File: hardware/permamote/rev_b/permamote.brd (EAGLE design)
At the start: 27 x 60 mm, 126 parts, among them J1 TC2030-JLINK-NL, J5 MICRO_USB_B_HIROSE_ZX62R-B-5P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, Q1 PMDXB950UPEL, Q10 PMDXB950UPEL, Q2 PMDXB950UPEL, Q3 PMDXB950UPEL, Q4 PMDXB950UPEL, Q5 PMDXB950UPEL, Q6 PMDXB950UPEL, Q7 PMDXB950UPEL, Q8 PMDXB950UPEL, U1 AB1815-T3, U10 NRF52840, U11 SI7021-A20-GM1, U12 TCS34725, U2 BQ25505, U3 EKMB1101111, U4 FT232RQ, U6 LIS2DW12, U7 MAX17222, U8 MAX44009, U9 MS5637-02BA03, X1 32MHz, X3 32.768kHz, X4 ABS07-32.768KHZ-7-T

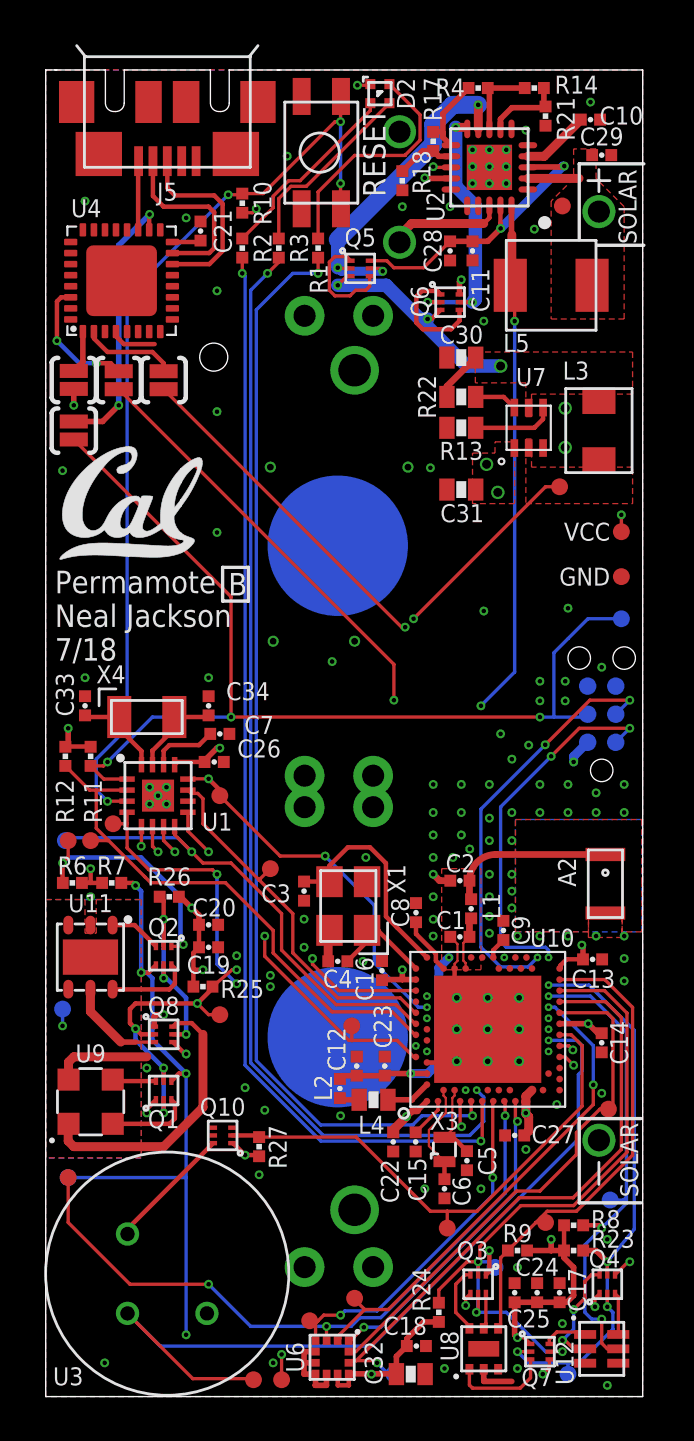
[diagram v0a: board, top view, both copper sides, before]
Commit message: Revert "Move jtag connector to back"
This reverts commit 0289d5f44ae80c2e7a408d73da812219b95e3e35.

start rev c
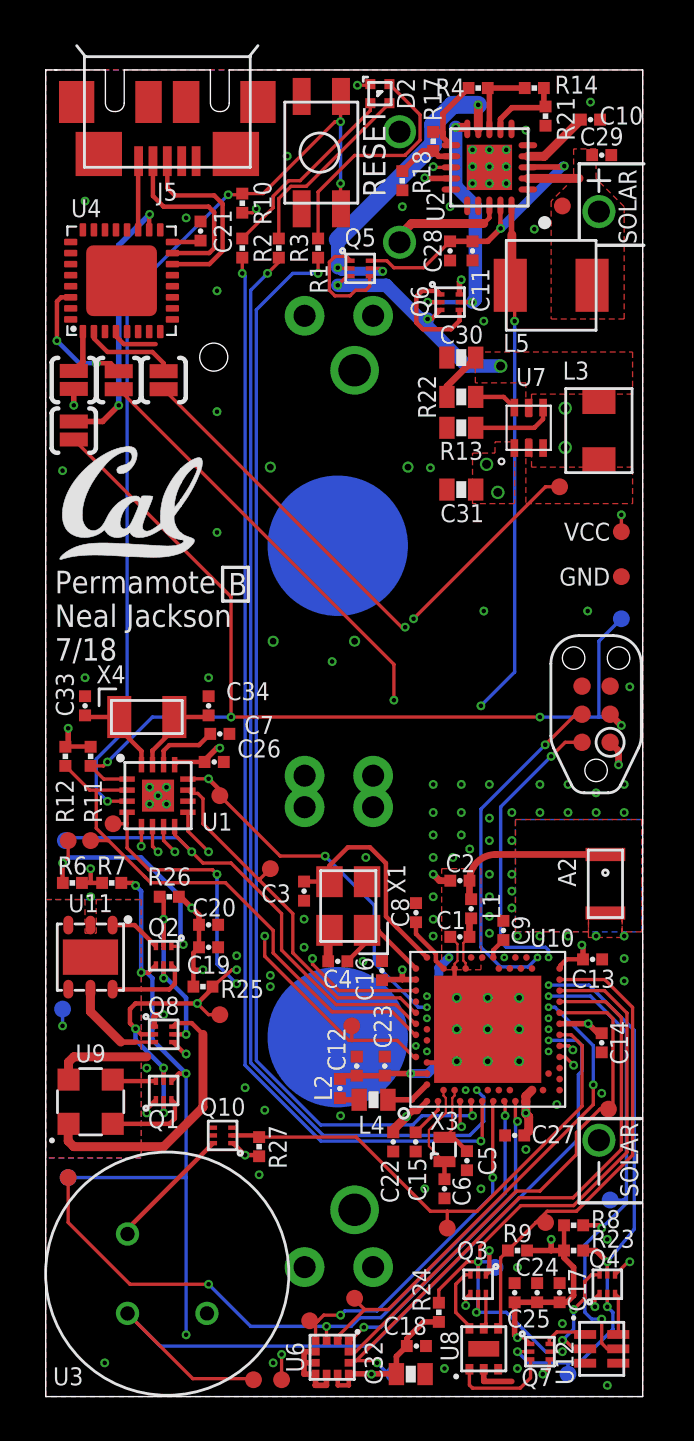
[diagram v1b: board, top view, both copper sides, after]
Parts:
- moved J1 0.25 mm to (24.9, 30.9), flipped to the top
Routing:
- net SWDCLK: track 19.0 -> 15.7 mm, vias 3 -> 2
- net SWDIO: track 17.0 -> 13.6 mm, vias 3 -> 2
- net !RST: track 64.9 -> 65.5 mm, vias 4 -> 5
- net GND: vias 117 -> 110
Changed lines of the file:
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@@
 <attribute name="NAME" x="7.62" y="21.717" size="0.8128" layer="25" font="vector" ratio="12" align="bottom-center"/>
 </element>
-<element name="J1" library="connector" package="TC2030-IDC-NL" value="TC2030-JLINK-NL" x="25.146" y="30.861" smashed="yes" rot="MR90">
-<attribute name="VALUE" x="19.1135" y="30.861" size="1.016" layer="28" font="vector" ratio="12" rot="MR90" align="bottom-center"/>
+<element name="J1" library="connector" package="TC2030-IDC-NL" value="TC2030-JLINK-NL" x="24.892" y="30.861" smashed="yes" rot="R90">
+<attribute name="VALUE" x="30.9245" y="30.861" size="1.016" layer="27" font="vector" ratio="12" rot="R90" align="bottom-center"/>
 </element>
 <element name="R23" library="passives" package="0402_RES" value="100M" x="23.876" y="6.604" smashed="yes" rot="R180">
@@
 <wire x1="17.242" y1="14.61" x2="16.51" y2="14.61" width="0.254" layer="1"/>
 <wire x1="16.51" y1="14.61" x2="15.43106875" y2="14.61" width="0.254" layer="1"/>
+<wire x1="18.242" y1="19.86" x2="18.2279625" y2="19.8740375" width="0.2032" layer="1"/>
 <via x="16.51" y="14.61" extent="1-16" drill="0.2032"/>
 <via x="18.242" y="19.86" extent="1-16" drill="0.1524"/>
@@
 <contactref element="C21" pad="2"/>
 <contactref element="J5" pad="5"/>
+<wire x1="18.534" y1="18.6392" x2="18.5288" y2="18.634" width="0.1016" layer="1"/>
 <via x="18.288" y="53.816" extent="1-16" drill="0.2032"/>
 <via x="6.35" y="53.308" extent="1-16" drill="0.2032"/>
@@
 <wire x1="3.18" y1="47.95599375" x2="3.53639375" y2="47.5996" width="0.2032" layer="1"/>
 <wire x1="3.18" y1="48.167" x2="3.18" y2="47.95599375" width="0.2032" layer="1"/>
+<wire x1="3.53639375" y1="47.5996" x2="4.9733" y2="47.5996" width="0.2032" layer="1"/>
 <via x="11.684" y="21.59" extent="1-16" drill="0.2032"/>
 <via x="11.684" y="20.32" extent="1-16" drill="0.2032"/>
@@
 <via x="17.399" y="42.005" extent="1-16" drill="0.2032"/>
 <via x="19.812" y="35.528" extent="1-16" drill="0.2032"/>
-<via x="23.622" y="35.655" extent="1-16" drill="0.2032"/>
-<via x="23.495" y="32.353" extent="1-16" drill="0.2032"/>
+<via x="24.511" y="35.528" extent="1-16" drill="0.2032"/>
+<via x="26.416" y="32.099" extent="1-16" drill="0.2032"/>
 <contactref element="C9" pad="2"/>
 <via x="21.336" y="20.828" extent="1-16" drill="0.2032"/>
@@
 <wire x1="17.526" y1="23.622" x2="17.815" y2="23.333" width="0.3048" layer="1"/>
 <wire x1="17.815" y1="23.333" x2="18.29893125" y2="23.333" width="0.3048" layer="1"/>
-<via x="23.495" y="31.464" extent="1-16" drill="0.2032"/>
-<via x="25.146" y="32.988" extent="1-16" drill="0.2032"/>
-<via x="22.352" y="32.353" extent="1-16" drill="0.2032"/>
-<via x="22.352" y="31.464" extent="1-16" drill="0.2032"/>
-<wire x1="3.53639375" y1="47.5996" x2="4.9276" y2="47.5996" width="0.2032" layer="1"/>
-<via x="21.082" y="28.829" extent="1-16" drill="0.2032"/>
-<via x="21.844" y="29.464" extent="1-16" drill="0.2032"/>
-<via x="20.574" y="29.972" extent="1-16" drill="0.2032"/>
 </signal>
 <signal name="N$8">
@@
 <wire x1="6.93293125" y1="21.336" x2="6.93293125" y2="21.76906875" width="0.254" layer="1"/>
 <wire x1="6.93293125" y1="21.76906875" x2="6.604" y2="22.098" width="0.254" layer="1"/>
-<via x="23.876" y="28.702" extent="1-16" drill="0.2032"/>
+<via x="25.908" y="28.575" extent="1-16" drill="0.2032"/>
 <wire x1="16.129" y1="19.304" x2="16.129" y2="18.86" width="0.254" layer="1"/>
 <wire x1="16.33093125" y1="2.286" x2="16.33093125" y2="2.61493125" width="0.254" layer="1"/>
@@
 <wire x1="13.97" y1="34.163" x2="15.748" y2="34.163" width="0.8128" layer="15"/>
 <via x="10.287" y="34.163" extent="1-16" drill="0.3048"/>
+<wire x1="25.908" y1="28.575" x2="25.908" y2="29.21" width="0.3048" layer="1"/>
+<wire x1="25.908" y1="29.21" x2="25.527" y2="29.591" width="0.3048" layer="1"/>
 <wire x1="15.748" y1="34.163" x2="16.383" y2="33.528" width="0.8128" layer="15"/>
-<wire x1="24.511" y1="29.591" x2="23.876" y2="28.956" width="0.4064" layer="16"/>
-<wire x1="23.876" y1="28.956" x2="23.876" y2="28.702" width="0.4064" layer="16"/>
+<wire x1="16.383" y1="33.528" x2="16.4338" y2="33.528" width="0.8128" layer="15"/>
 </signal>
 <signal name="N$12">
@@
 <via x="22.742" y="16.61" extent="1-16" drill="0.1524"/>
 <contactref element="SJ3" pad="1"/>
+<via x="26.035" y="30.353" extent="1-16" drill="0.2032"/>
 <wire x1="2.032" y1="28.52293125" x2="2.62693125" y2="27.928" width="0.1524" layer="1"/>
 <wire x1="2.62693125" y1="27.928" x2="3.68" y2="27.928" width="0.1524" layer="1"/>
@@
 <wire x1="1.27" y1="43.2871" x2="8.382" y2="36.1751" width="0.1524" layer="1"/>
 <wire x1="8.382" y1="36.1751" x2="8.382" y2="30.734" width="0.1524" layer="1"/>
+<wire x1="26.035" y1="35.179" x2="25.019" y2="34.163" width="0.1524" layer="16"/>
+<wire x1="25.527" y1="30.861" x2="26.035" y2="30.353" width="0.3048" layer="1"/>
+<wire x1="22.352" y1="30.734" x2="25.019" y2="30.734" width="0.1524" layer="16"/>
+<wire x1="25.019" y1="30.734" x2="25.654" y2="30.734" width="0.1524" layer="16"/>
+<wire x1="25.654" y1="30.734" x2="26.035" y2="30.353" width="0.1524" layer="16"/>
+<wire x1="25.019" y1="34.163" x2="25.019" y2="30.734" width="0.1524" layer="16"/>
 <wire x1="22.742" y1="16.61" x2="22.91" y2="16.61" width="0.1524" layer="15"/>
-<wire x1="22.352" y1="30.734" x2="22.987" y2="30.734" width="0.1524" layer="16"/>
-<wire x1="22.987" y1="30.734" x2="24.384" y2="30.734" width="0.1524" layer="16"/>
-<wire x1="24.384" y1="30.734" x2="24.511" y2="30.861" width="0.1524" layer="16"/>
-<wire x1="22.987" y1="33.6422375" x2="23.6347625" y2="34.29" width="0.1524" layer="16"/>
-<wire x1="22.987" y1="30.734" x2="22.987" y2="33.6422375" width="0.1524" layer="16"/>
-<wire x1="23.6347625" y1="34.29" x2="24.5237625" y2="35.179" width="0.1524" layer="16"/>
-<wire x1="24.5237625" y1="35.179" x2="26.035" y2="35.179" width="0.1524" layer="16"/>
 </signal>
 <signal name="!RTC_IRQ1">
@@
 <wire x1="20.574" y1="26.67" x2="20.574" y2="20.574" width="0.1524" layer="16"/>
 <wire x1="20.574" y1="20.574" x2="20.828" y2="20.32" width="0.1524" layer="16"/>
-<wire x1="22.86" y1="28.956" x2="24.13" y2="30.226" width="0.1524" layer="1"/>
-<wire x1="24.13" y1="30.226" x2="26.416" y2="30.226" width="0.1524" layer="1"/>
-<via x="26.416" y="30.226" extent="1-16" drill="0.2032"/>
-<wire x1="26.416" y1="30.226" x2="25.781" y2="29.591" width="0.1524" layer="16"/>
+<wire x1="22.86" y1="28.956" x2="23.495" y2="29.591" width="0.1524" layer="1"/>
+<wire x1="23.495" y1="29.591" x2="24.257" y2="29.591" width="0.1524" layer="1"/>
 </signal>
 <signal name="RTC_CS">
@@
 <wire x1="19.685" y1="20.32" x2="19.685" y2="26.57126875" width="0.1524" layer="16"/>
 <wire x1="19.685" y1="26.57126875" x2="22.591865625" y2="29.478134375" width="0.1524" layer="16"/>
-<wire x1="22.591865625" y1="29.478134375" x2="24.60973125" y2="31.496" width="0.1524" layer="1"/>
-<wire x1="24.60973125" y1="31.496" x2="26.416" y2="31.496" width="0.1524" layer="1"/>
-<via x="26.416" y="31.496" extent="1-16" drill="0.2032"/>
-<wire x1="26.416" y1="31.496" x2="25.781" y2="30.861" width="0.1524" layer="16"/>
+<wire x1="22.591865625" y1="29.478134375" x2="23.97473125" y2="30.861" width="0.1524" layer="1"/>
+<wire x1="23.97473125" y1="30.861" x2="24.257" y2="30.861" width="0.1524" layer="1"/>
 </signal>
 <signal name="N$41">

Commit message: Move jtag connector to back
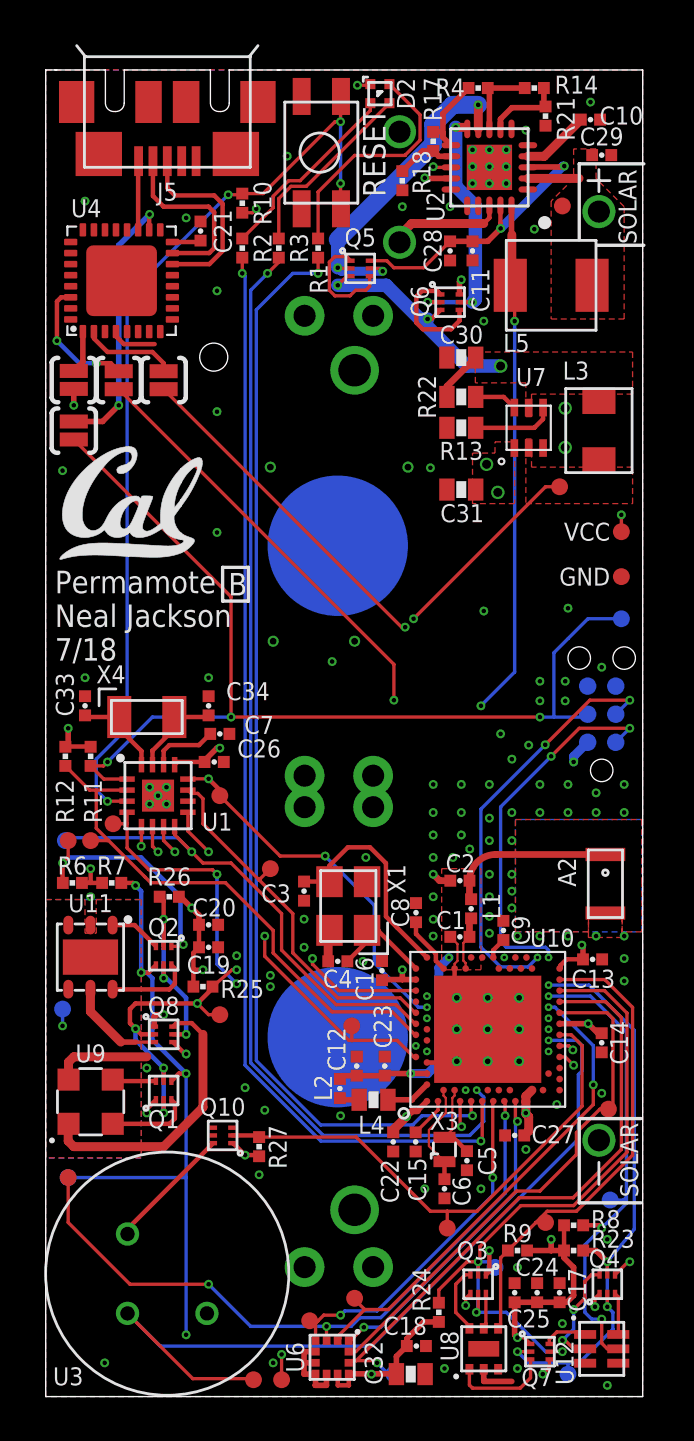
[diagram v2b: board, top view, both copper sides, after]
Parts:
- moved J1 0.25 mm to (25.1, 30.9), flipped to the bottom
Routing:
- net SWDCLK: track 15.7 -> 19.0 mm, vias 2 -> 3
- net SWDIO: track 13.6 -> 17.0 mm, vias 2 -> 3
- net !RST: track 65.5 -> 64.9 mm, vias 5 -> 4
- net GND: vias 110 -> 117
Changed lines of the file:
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@@
 <attribute name="NAME" x="7.62" y="21.717" size="0.8128" layer="25" font="vector" ratio="12" align="bottom-center"/>
 </element>
-<element name="J1" library="connector" package="TC2030-IDC-NL" value="TC2030-JLINK-NL" x="24.892" y="30.861" smashed="yes" rot="R90">
-<attribute name="VALUE" x="30.9245" y="30.861" size="1.016" layer="27" font="vector" ratio="12" rot="R90" align="bottom-center"/>
+<element name="J1" library="connector" package="TC2030-IDC-NL" value="TC2030-JLINK-NL" x="25.146" y="30.861" smashed="yes" rot="MR90">
+<attribute name="VALUE" x="19.1135" y="30.861" size="1.016" layer="28" font="vector" ratio="12" rot="MR90" align="bottom-center"/>
 </element>
 <element name="R23" library="passives" package="0402_RES" value="100M" x="23.876" y="6.604" smashed="yes" rot="R180">
@@
 <wire x1="17.242" y1="14.61" x2="16.51" y2="14.61" width="0.254" layer="1"/>
 <wire x1="16.51" y1="14.61" x2="15.43106875" y2="14.61" width="0.254" layer="1"/>
-<wire x1="18.242" y1="19.86" x2="18.2279625" y2="19.8740375" width="0.2032" layer="1"/>
 <via x="16.51" y="14.61" extent="1-16" drill="0.2032"/>
 <via x="18.242" y="19.86" extent="1-16" drill="0.1524"/>
@@
 <contactref element="C21" pad="2"/>
 <contactref element="J5" pad="5"/>
-<wire x1="18.534" y1="18.6392" x2="18.5288" y2="18.634" width="0.1016" layer="1"/>
 <via x="18.288" y="53.816" extent="1-16" drill="0.2032"/>
 <via x="6.35" y="53.308" extent="1-16" drill="0.2032"/>
@@
 <wire x1="3.18" y1="47.95599375" x2="3.53639375" y2="47.5996" width="0.2032" layer="1"/>
 <wire x1="3.18" y1="48.167" x2="3.18" y2="47.95599375" width="0.2032" layer="1"/>
-<wire x1="3.53639375" y1="47.5996" x2="4.9733" y2="47.5996" width="0.2032" layer="1"/>
 <via x="11.684" y="21.59" extent="1-16" drill="0.2032"/>
 <via x="11.684" y="20.32" extent="1-16" drill="0.2032"/>
@@
 <via x="17.399" y="42.005" extent="1-16" drill="0.2032"/>
 <via x="19.812" y="35.528" extent="1-16" drill="0.2032"/>
-<via x="24.511" y="35.528" extent="1-16" drill="0.2032"/>
-<via x="26.416" y="32.099" extent="1-16" drill="0.2032"/>
+<via x="23.622" y="35.655" extent="1-16" drill="0.2032"/>
+<via x="23.495" y="32.353" extent="1-16" drill="0.2032"/>
 <contactref element="C9" pad="2"/>
 <via x="21.336" y="20.828" extent="1-16" drill="0.2032"/>
@@
 <wire x1="17.526" y1="23.622" x2="17.815" y2="23.333" width="0.3048" layer="1"/>
 <wire x1="17.815" y1="23.333" x2="18.29893125" y2="23.333" width="0.3048" layer="1"/>
+<via x="23.495" y="31.464" extent="1-16" drill="0.2032"/>
+<via x="25.146" y="32.988" extent="1-16" drill="0.2032"/>
+<via x="22.352" y="32.353" extent="1-16" drill="0.2032"/>
+<via x="22.352" y="31.464" extent="1-16" drill="0.2032"/>
+<wire x1="3.53639375" y1="47.5996" x2="4.9276" y2="47.5996" width="0.2032" layer="1"/>
+<via x="21.082" y="28.829" extent="1-16" drill="0.2032"/>
+<via x="21.844" y="29.464" extent="1-16" drill="0.2032"/>
+<via x="20.574" y="29.972" extent="1-16" drill="0.2032"/>
 </signal>
 <signal name="N$8">
@@
 <wire x1="6.93293125" y1="21.336" x2="6.93293125" y2="21.76906875" width="0.254" layer="1"/>
 <wire x1="6.93293125" y1="21.76906875" x2="6.604" y2="22.098" width="0.254" layer="1"/>
-<via x="25.908" y="28.575" extent="1-16" drill="0.2032"/>
+<via x="23.876" y="28.702" extent="1-16" drill="0.2032"/>
 <wire x1="16.129" y1="19.304" x2="16.129" y2="18.86" width="0.254" layer="1"/>
 <wire x1="16.33093125" y1="2.286" x2="16.33093125" y2="2.61493125" width="0.254" layer="1"/>
@@
 <wire x1="13.97" y1="34.163" x2="15.748" y2="34.163" width="0.8128" layer="15"/>
 <via x="10.287" y="34.163" extent="1-16" drill="0.3048"/>
-<wire x1="25.908" y1="28.575" x2="25.908" y2="29.21" width="0.3048" layer="1"/>
-<wire x1="25.908" y1="29.21" x2="25.527" y2="29.591" width="0.3048" layer="1"/>
 <wire x1="15.748" y1="34.163" x2="16.383" y2="33.528" width="0.8128" layer="15"/>
-<wire x1="16.383" y1="33.528" x2="16.4338" y2="33.528" width="0.8128" layer="15"/>
+<wire x1="24.511" y1="29.591" x2="23.876" y2="28.956" width="0.4064" layer="16"/>
+<wire x1="23.876" y1="28.956" x2="23.876" y2="28.702" width="0.4064" layer="16"/>
 </signal>
 <signal name="N$12">
@@
 <via x="22.742" y="16.61" extent="1-16" drill="0.1524"/>
 <contactref element="SJ3" pad="1"/>
-<via x="26.035" y="30.353" extent="1-16" drill="0.2032"/>
 <wire x1="2.032" y1="28.52293125" x2="2.62693125" y2="27.928" width="0.1524" layer="1"/>
 <wire x1="2.62693125" y1="27.928" x2="3.68" y2="27.928" width="0.1524" layer="1"/>
@@
 <wire x1="1.27" y1="43.2871" x2="8.382" y2="36.1751" width="0.1524" layer="1"/>
 <wire x1="8.382" y1="36.1751" x2="8.382" y2="30.734" width="0.1524" layer="1"/>
-<wire x1="26.035" y1="35.179" x2="25.019" y2="34.163" width="0.1524" layer="16"/>
-<wire x1="25.527" y1="30.861" x2="26.035" y2="30.353" width="0.3048" layer="1"/>
-<wire x1="22.352" y1="30.734" x2="25.019" y2="30.734" width="0.1524" layer="16"/>
-<wire x1="25.019" y1="30.734" x2="25.654" y2="30.734" width="0.1524" layer="16"/>
-<wire x1="25.654" y1="30.734" x2="26.035" y2="30.353" width="0.1524" layer="16"/>
-<wire x1="25.019" y1="34.163" x2="25.019" y2="30.734" width="0.1524" layer="16"/>
 <wire x1="22.742" y1="16.61" x2="22.91" y2="16.61" width="0.1524" layer="15"/>
+<wire x1="22.352" y1="30.734" x2="22.987" y2="30.734" width="0.1524" layer="16"/>
+<wire x1="22.987" y1="30.734" x2="24.384" y2="30.734" width="0.1524" layer="16"/>
+<wire x1="24.384" y1="30.734" x2="24.511" y2="30.861" width="0.1524" layer="16"/>
+<wire x1="22.987" y1="33.6422375" x2="23.6347625" y2="34.29" width="0.1524" layer="16"/>
+<wire x1="22.987" y1="30.734" x2="22.987" y2="33.6422375" width="0.1524" layer="16"/>
+<wire x1="23.6347625" y1="34.29" x2="24.5237625" y2="35.179" width="0.1524" layer="16"/>
+<wire x1="24.5237625" y1="35.179" x2="26.035" y2="35.179" width="0.1524" layer="16"/>
 </signal>
 <signal name="!RTC_IRQ1">
@@
 <wire x1="20.574" y1="26.67" x2="20.574" y2="20.574" width="0.1524" layer="16"/>
 <wire x1="20.574" y1="20.574" x2="20.828" y2="20.32" width="0.1524" layer="16"/>
-<wire x1="22.86" y1="28.956" x2="23.495" y2="29.591" width="0.1524" layer="1"/>
-<wire x1="23.495" y1="29.591" x2="24.257" y2="29.591" width="0.1524" layer="1"/>
+<wire x1="22.86" y1="28.956" x2="24.13" y2="30.226" width="0.1524" layer="1"/>
+<wire x1="24.13" y1="30.226" x2="26.416" y2="30.226" width="0.1524" layer="1"/>
+<via x="26.416" y="30.226" extent="1-16" drill="0.2032"/>
+<wire x1="26.416" y1="30.226" x2="25.781" y2="29.591" width="0.1524" layer="16"/>
 </signal>
 <signal name="RTC_CS">
@@
 <wire x1="19.685" y1="20.32" x2="19.685" y2="26.57126875" width="0.1524" layer="16"/>
 <wire x1="19.685" y1="26.57126875" x2="22.591865625" y2="29.478134375" width="0.1524" layer="16"/>
-<wire x1="22.591865625" y1="29.478134375" x2="23.97473125" y2="30.861" width="0.1524" layer="1"/>
-<wire x1="23.97473125" y1="30.861" x2="24.257" y2="30.861" width="0.1524" layer="1"/>
+<wire x1="22.591865625" y1="29.478134375" x2="24.60973125" y2="31.496" width="0.1524" layer="1"/>
+<wire x1="24.60973125" y1="31.496" x2="26.416" y2="31.496" width="0.1524" layer="1"/>
+<via x="26.416" y="31.496" extent="1-16" drill="0.2032"/>
+<wire x1="26.416" y1="31.496" x2="25.781" y2="30.861" width="0.1524" layer="16"/>
 </signal>
 <signal name="N$41">
